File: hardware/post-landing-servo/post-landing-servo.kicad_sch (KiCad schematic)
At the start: 9 parts, among them J10 DE9_Socket, J6 Conn_01x06, J7 Conn_01x08, J8 Conn_01x08, J9 DE9_Socket

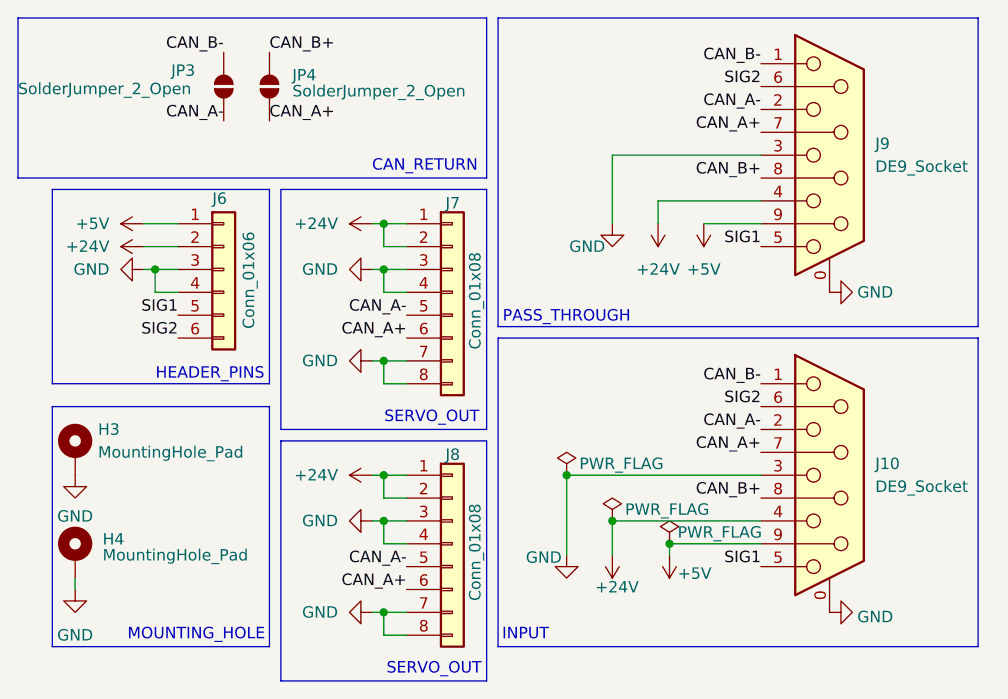
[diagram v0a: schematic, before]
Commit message: Feat: Reroute and minor fixes
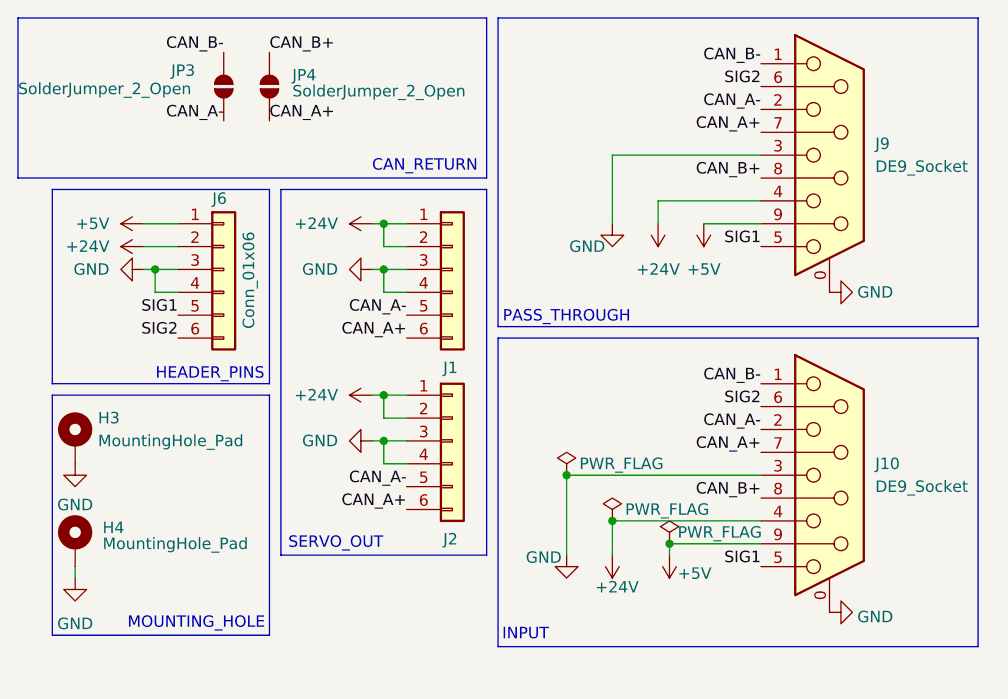
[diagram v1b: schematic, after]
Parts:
- removed J7, J8: Conn_01x08, Custom:ZH-6PWB_knockoff, symbol Connector_Generic:Conn_01x08
- added J1, J2: Conn_01x06, Connector_JST:JST_ZH_B6B-ZR-SM4-TF_1x06-1MP_P1.50mm_Vertical, symbol Connector_Generic:Conn_01x06
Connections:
- net +24V: now also J1.1 (Pin_1), J1.2 (Pin_2), J2.1 (Pin_1), J2.2 (Pin_2)
- net CAN_A+: now also J1.6 (Pin_6), J2.6 (Pin_6)
- net CAN_A-: now also J1.5 (Pin_5), J2.5 (Pin_5)
- net GND: now also J1.3 (Pin_3), J1.4 (Pin_4), J2.3 (Pin_3), J2.4 (Pin_4)
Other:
- moved on the sheet: H3, H4
